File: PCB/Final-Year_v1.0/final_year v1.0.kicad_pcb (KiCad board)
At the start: 2 copper layers, 37 parts, among them J1 Power In, J2 Screw_Terminal_01x07, J3 Screw_Terminal_01x03, J4 Screw_Terminal_01x04, J5 Screw_Terminal_01x03, J6 PT1000, J7 HCPV 22x, J8 LDR, J9 Screw_Terminal_01x03, U1 LM7805_TO220, U2 TL431LP, U4 ESP32-DEVKIT-V1, U5 LM324, U6 1085

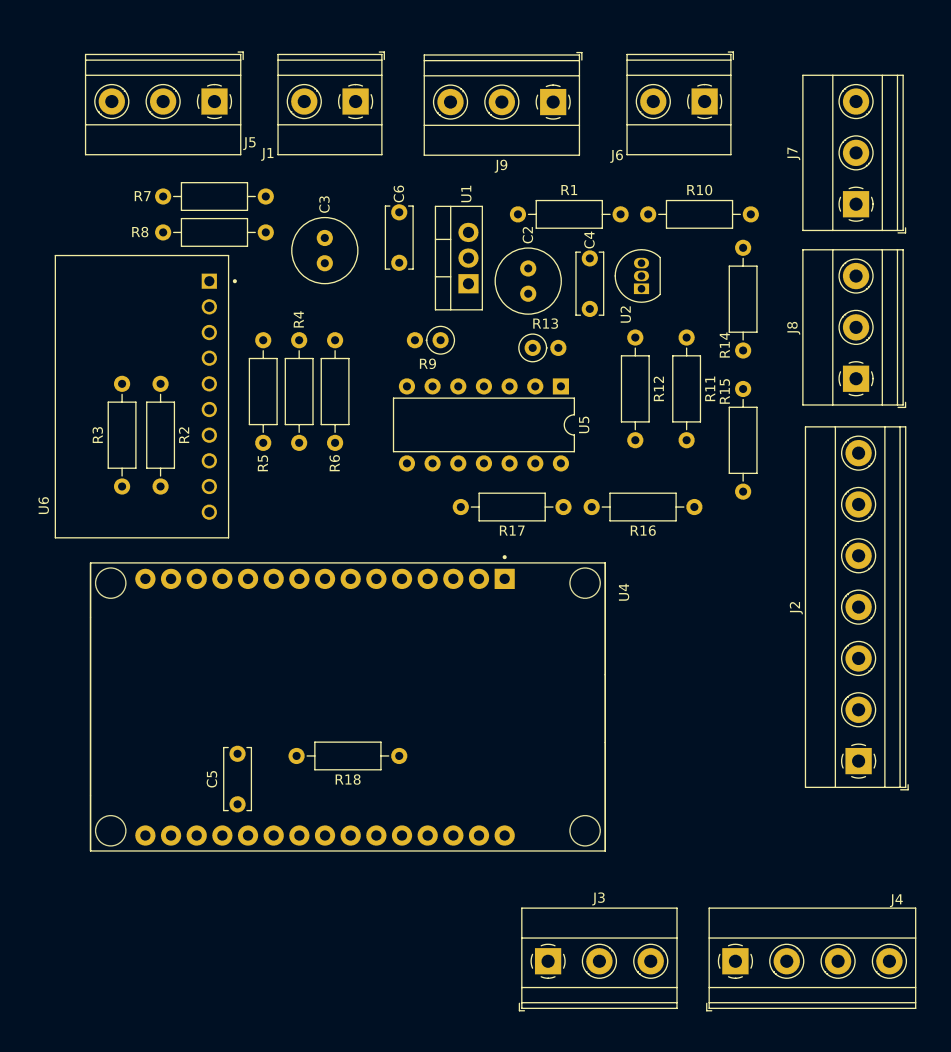
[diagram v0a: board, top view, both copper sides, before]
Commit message: Add files via upload
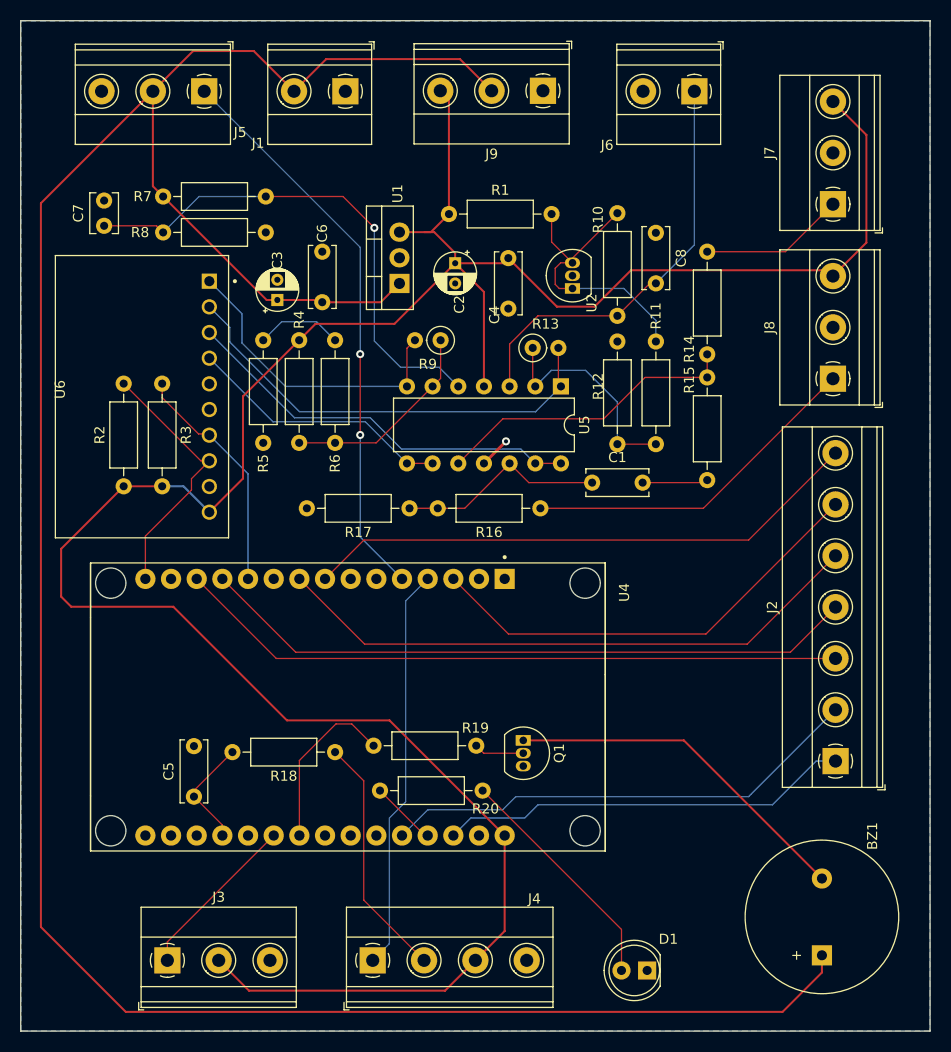
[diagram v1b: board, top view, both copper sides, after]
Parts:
- added BZ1: Buzzer, Buzzer_Beeper:Buzzer_15x7.5RM7.6, F.Cu at (91.4, 104.6)
- added C1: 0.1u, Capacitor_THT:C_Disc_D6.0mm_W2.5mm_P5.00mm, F.Cu at (68.6, 57.8)
- added C7: 10nF, Capacitor_THT:C_Disc_D3.8mm_W2.6mm_P2.50mm, F.Cu at (20.3, 32.4)
- added C8: 0.1uF, Capacitor_THT:C_Disc_D6.0mm_W2.5mm_P5.00mm, F.Cu at (74.9, 33.1)
- added D1: LED, LED_THT:LED_D5.0mm, F.Cu at (74.1, 106.1)
- added Q1: BC547, Package_TO_SOT_THT:TO-92_Inline, F.Cu at (61.8, 83.3)
- added R19: 1.2k, Resistor_THT:R_Axial_DIN0207_L6.3mm_D2.5mm_P10.16mm_Horizontal, F.Cu at (57.1, 83.8)
- added R20: 330, Resistor_THT:R_Axial_DIN0207_L6.3mm_D2.5mm_P10.16mm_Horizontal, F.Cu at (47.6, 88.3)
- C2: footprint Capacitor_THT:C_Radial_D6.3mm_H7.0mm_P2.50mm -> Capacitor_THT:CP_Radial_D4.0mm_P2.00mm
- C3: footprint Capacitor_THT:C_Radial_D6.3mm_H5.0mm_P2.50mm -> Capacitor_THT:CP_Radial_D4.0mm_P2.00mm
- J5: value Screw_Terminal_01x03 -> Actuator
- moved J3 37.7 mm to (26.6, 105.1)
- moved J4 35.9 mm to (46.9, 105.1)
- moved R17 15.2 mm to (50.5, 60.3)
- moved R16 15.2 mm to (63.5, 60.3)
- moved R3 10.9 mm to (26.1, 48.0), turned to -90 degrees
- moved R2 10.8 mm to (22.3, 58.1), turned to 90 degrees
- moved C6 8.56 mm to (41.9, 39.9)
- moved C4 8.07 mm to (60.3, 35.6)
- moved C2 7.25 mm to (55.1, 36.1)
- moved U2 6.83 mm to (66.7, 38.6)
- moved R1 6.83 mm to (54.4, 31.2)
- moved U1 6.83 mm to (49.6, 38.1)
- moved R18 6.36 mm to (43.2, 84.5)
- moved C3 5.94 mm to (37.5, 39.7)
- moved C5 4.38 mm to (29.2, 88.9)
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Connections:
- J2 pad 1: TX0 -> D13
- J2 pad 2: RX0 -> D14
- J2 pad 3: D18 -> TX0
- J2 pad 4: D15 -> RX0
- J2 pad 5: D14 -> D18
- J2 pad 6: D13 -> D15
- U4 pad 22: unconnected-(U4-D33-Pad22) -> D33
- U4 pad 27: unconnected-(U4-D12-Pad27) -> D12
- U6 pad 1: LDR -> Battery_level
- U6 pad 2: Battery_level -> PT1000
- U6 pad 3: HCPV -> LDR
- U6 pad 4: PT1000 -> HCPV
- U6 pad 6: unconnected-(U6-ADDR-Pad6) -> GND
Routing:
- net +5V: track 0.00 -> 255.2 mm
- net +12V: track 0.00 -> 250.2 mm
- net TX0: track 0.00 -> 66.5 mm
- net RX0: track 0.00 -> 65.5 mm
- net D18: track 0.00 -> 59.4 mm
- net D4: track 0.00 -> 56.4 mm, vias 0 -> 2
- net D5: track 0.00 -> 55.7 mm
- net Net-(U5B-+): track 0.00 -> 51.1 mm, vias 0 -> 1
- net D14: track 0.00 -> 48.1 mm
- net D15: track 0.00 -> 45.4 mm
- net PT1000: track 0.00 -> 44.9 mm
- net Net-(J6-Pin_1): track 0.00 -> 41.7 mm
- net D13: track 0.00 -> 40.9 mm
- net LDR: track 0.00 -> 40.2 mm
- net D2: track 0.00 -> 40.0 mm
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- added copper zone on B.Cu, net GND
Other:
- board outline added: 90 x 100 mm
